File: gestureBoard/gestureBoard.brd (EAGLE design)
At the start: 10.1 x 13.6 mm, 11 parts, among them J1 GRPB042MWCN-RC, U1 APDS-9960

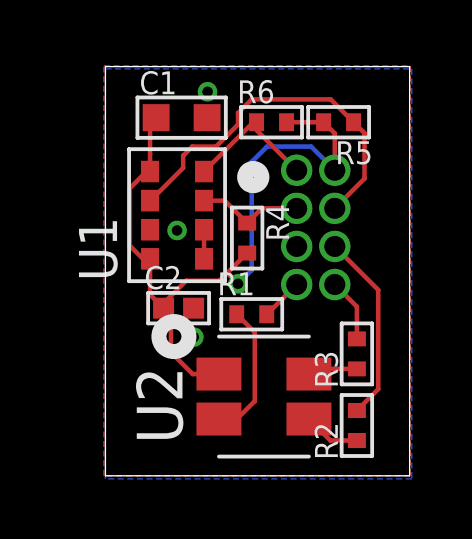
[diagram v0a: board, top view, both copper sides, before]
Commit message: more progress on routing
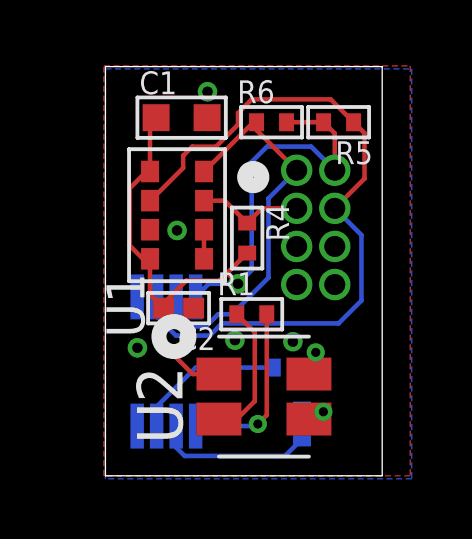
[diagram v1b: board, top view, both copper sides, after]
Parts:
- added U3: PCA9553TSSOP8, glasses:SOP65P490X110-8
- moved R3 2.33 mm to (6.10, 3.61), flipped to the bottom, turned to 0 degrees
- moved R2 1.83 mm to (6.55, 1.73), flipped to the bottom, turned to 270 degrees
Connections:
- net +3V3: now also U3.8
- net GND: now also U3.4
- net LED_B: now also U3.3; no longer J1.4
- net LED_G: now also U3.2; no longer J1.3
- net LED_R: now also U3.1; no longer J1.5
- net SCL: now also U3.6
- net SDA: now also U3.7
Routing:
- net SCL: track 12.4 -> 24.1 mm
- net SDA: track 4.58 -> 13.1 mm
- net LED_R: track 1.41 -> 5.88 mm, vias 0 -> 1
- net LED_B: track 2.12 -> 5.08 mm
- net +3V3: track 25.6 -> 27.2 mm
- net LED_G: track 6.36 -> 5.26 mm
- net N$2: track 1.90 -> 1.33 mm, vias 0 -> 1
- net N$3: track 1.67 -> 1.50 mm, vias 0 -> 1
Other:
- board size 10.1 x 13.6 mm -> 9.2 x 13.6 mm
